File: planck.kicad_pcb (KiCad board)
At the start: 2 copper layers, 113 x 75 mm, 54 parts, among them J1 USB_C_U262-161N-4BVC11, J2 USB_C_U262-161N-4BVC11, SW1 SW_Cherry_MX_1.00u, SW10 SW_Cherry_MX_1.00u, SW11 SW_Cherry_MX_1.00u, SW12 SW_Cherry_MX_1.00u, SW13 SW_Cherry_MX_1.00u, SW14 SW_Cherry_MX_1.00u, SW15 SW_Cherry_MX_1.00u, SW16 SW_Cherry_MX_1.00u, SW17 SW_Cherry_MX_1.00u, SW18 SW_Cherry_MX_1.00u, SW19 SW_Cherry_MX_1.00u, SW2 SW_Cherry_MX_1.00u, SW20 SW_Cherry_MX_1.00u, SW21 SW_Cherry_MX_1.00u, SW22 SW_Cherry_MX_1.00u, SW23 SW_Cherry_MX_1.00u, SW24 SW_Cherry_MX_1.00u, SW3 SW_Cherry_MX_1.00u, SW4 SW_Cherry_MX_1.00u, SW5 SW_Cherry_MX_1.00u, SW6 SW_Cherry_MX_1.00u, SW7 SW_Cherry_MX_1.00u, SW8 SW_Cherry_MX_1.00u, SW9 SW_Cherry_MX_1.00u, U1 RP2040, Y1 32M

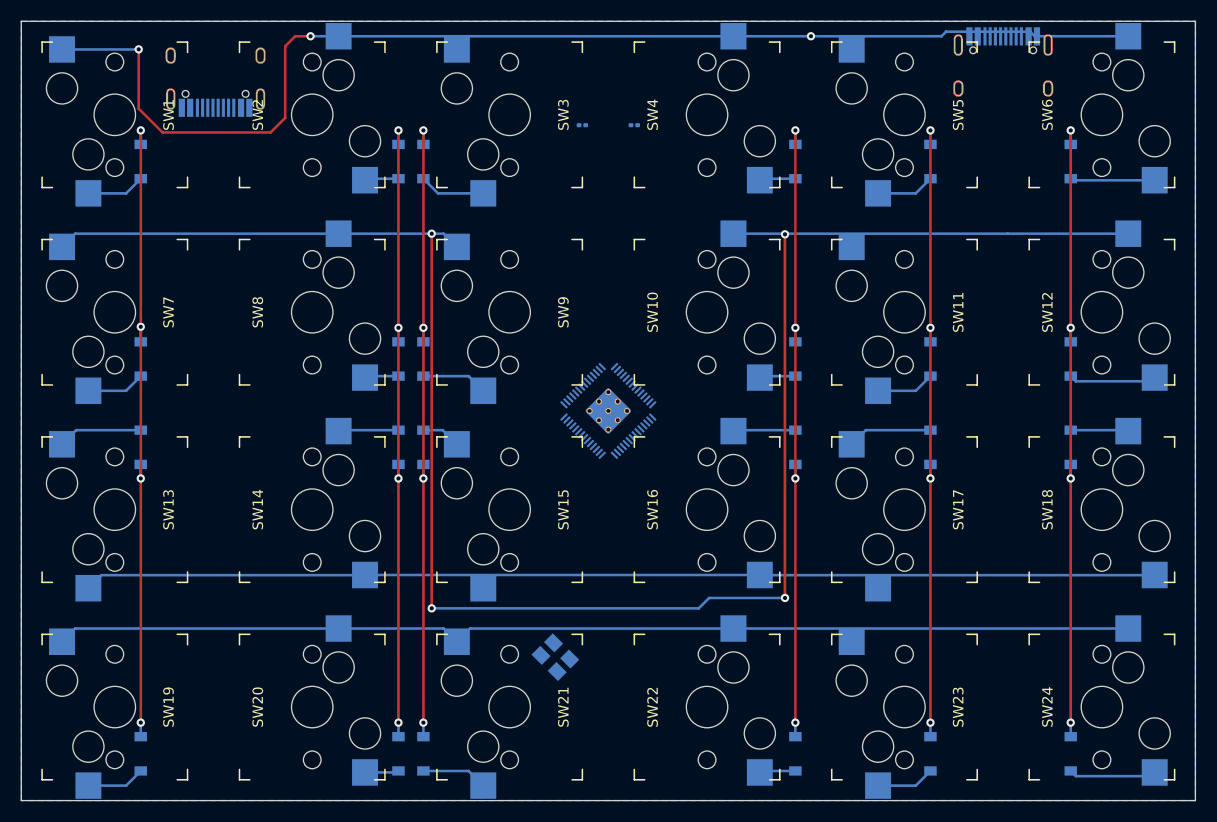
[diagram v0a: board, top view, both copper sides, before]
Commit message: MX version complete
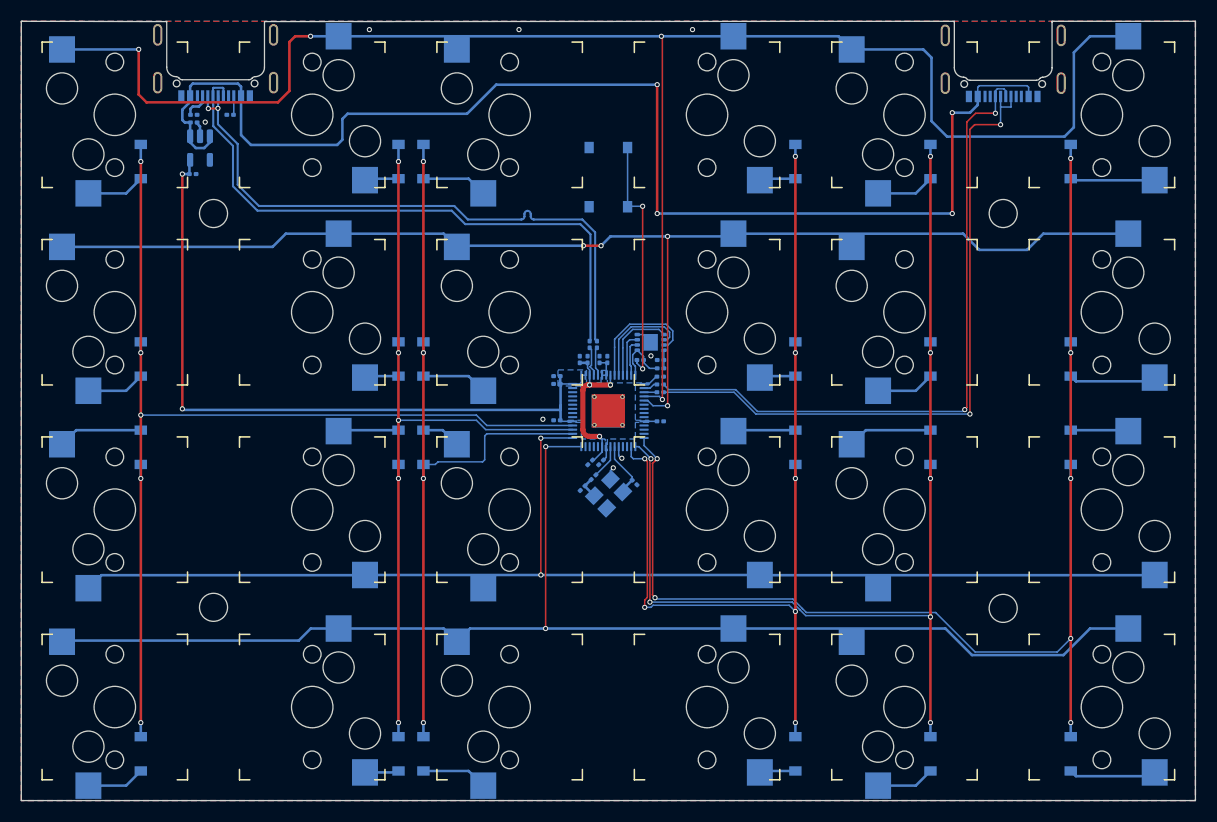
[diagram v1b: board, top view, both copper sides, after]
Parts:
- added C1: 2.2uF ±10% 10V, Resistor_SMD:R_0201_0603Metric, B.Cu at (99.1, 69.7)
- added C10: 100nF ±10% 25V 0201, Resistor_SMD:R_0201_0603Metric, B.Cu at (138.2, 92.5)
- added C11: 100nF ±10% 25V 0201, Resistor_SMD:R_0201_0603Metric, B.Cu at (144.0, 98.5)
- added C12: 100nF ±10% 25V 0201, Resistor_SMD:R_0201_0603Metric, B.Cu at (138.3, 102.5)
- added C13: 100nF ±10% 25V 0201, Resistor_SMD:R_0201_0603Metric, B.Cu at (138.9, 92.5)
- added C14: 1uF ±20% 6.3V 0201, Capacitor_SMD:C_0201_0603Metric, B.Cu at (137.0, 92.5)
- added C15: 100nF ±10% 25V 0201, Resistor_SMD:R_0201_0603Metric, B.Cu at (136.2, 92.5)
- added C16: 100nF ±10% 25V 0201, Resistor_SMD:R_0201_0603Metric, B.Cu at (137.2, 102.5)
- added C2: 2.2uF ±10% 10V, Resistor_SMD:R_0201_0603Metric, B.Cu at (99.0, 74.7)
- added C3: 22pF ±5% 50V 0603, Resistor_SMD:R_0201_0603Metric, B.Cu at (141.5, 104.4)
- added C4: 22pF ±5% 50V 0603, Resistor_SMD:R_0201_0603Metric, B.Cu at (136.5, 104.9)
- added C5: 100nF ±10% 25V 0201, Resistor_SMD:R_0201_0603Metric, B.Cu at (144.0, 92.6)
- added C6: 1uF ±20% 6.3V 0201, Capacitor_SMD:C_0201_0603Metric, B.Cu at (134.1, 94.2)
- added C7: 100nF ±10% 25V 0201, Resistor_SMD:R_0201_0603Metric, B.Cu at (134.1, 94.9)
- added C8: 100nF ±10% 25V 0201, Resistor_SMD:R_0201_0603Metric, B.Cu at (144.0, 94.2)
- added C9: 100nF ±10% 25V 0201, Resistor_SMD:R_0201_0603Metric, B.Cu at (134.1, 98.4)
- added H1: MountingHole, MountingHole:MountingHole_2.7mm_M2.5, F.Cu at (101.0, 78.5)
- added H2: MountingHole, MountingHole:MountingHole_2.7mm_M2.5, F.Cu at (177.0, 78.5)
- added H3: MountingHole, MountingHole:MountingHole_2.7mm_M2.5, F.Cu at (177.0, 116.5)
- added H4: MountingHole, MountingHole:MountingHole_2.7mm_M2.5, F.Cu at (101.0, 116.4)
- added R3: 1kΩ ±1% 50mW 0201, Resistor_SMD:R_0201_0603Metric, B.Cu at (137.6, 103.9)
- added R4: 100Ω ±1% 50mW, Resistor_SMD:R_0201_0603Metric, B.Cu at (144.0, 95.0)
- added R5: 27Ω ±1% 50mW 0201, Resistor_SMD:R_0201_0603Metric, B.Cu at (137.9, 91.1)
- added R6: 27Ω ±1% 50mW 0201, Resistor_SMD:R_0201_0603Metric, B.Cu at (137.2, 91.1)
- added R7: 100Ω ±1% 50mW, Resistor_SMD:R_0201_0603Metric, B.Cu at (144.0, 95.7)
- added R8: 10kΩ ±1% 50mW 0201, Resistor_SMD:R_0201_0603Metric, B.Cu at (144.0, 93.4)
- added R9: 1kΩ ±1% 50mW 0201, Resistor_SMD:R_0201_0603Metric, B.Cu at (142.1, 92.6)
- added SW25: SW_Push, Switches:TSC005A1618A03, B.Cu at (139.0, 75.0)
- added U2: ME6219C33M5G, Package_TO_SOT_SMD:SOT-23-5, B.Cu at (99.7, 72.2)
- added U3: W25Q16JVUXIQ, Package_SON:SON-8-1EP_3x2mm_P0.5mm_EP1.4x1.6mm, B.Cu at (143.1, 90.9)
- D1, D10, D11, D12, D13, D14, D15, D16, D17, D18, D19, D2, D20, D21, D22, D23, D24, D3, D4, D5, D6, D7, D8, D9: value 1N4148W -> 1N4148W,100V 150mA 4ns T4
- J1, J2: footprint josh-connectors:USB_C_U262-161N-4BVC11 -> josh-connectors:USB_C_TYPE-C-31-M-14
- U1: value RP2040 -> RP2040 ARM Cortex-M0 133MHz; footprint RP2040_minimal:RP2040-QFN-56 -> Package_DFN_QFN:QFN-56-1EP_7x7mm_P0.4mm_EP3.2x3.2mm_ThermalVias
- Y1: value 32M -> 32MHz ±10ppm 20pF SMD3225-4P
- moved R2 38.9 mm to (102.6, 69.0), turned to 180 degrees
- moved R1 37.4 mm to (99.1, 69.0), turned to 0 degrees
- moved Y1 16.5 mm to (139.0, 105.5), turned to -135 degrees
- moved J2 0.85 mm to (101.2, 64.3)
- moved J1 0.22 mm to (177.0, 64.4), turned to 0 degrees
- turned U1 to 180 degrees
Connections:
- net /d+ renamed /D-
- net /d- renamed /D+
- U1 pad 1: unconnected-(U1-Pad1) -> /V3V3
- U1 pad 10: unconnected-(U1-Pad10) -> /V3V3
- U1 pad 14: unconnected-(U1-Pad14) -> c6
- U1 pad 15: unconnected-(U1-Pad15) -> c5
- U1 pad 16: unconnected-(U1-Pad16) -> c4
- U1 pad 19: unconnected-(U1-Pad19) -> GND
- U1 pad 2: unconnected-(U1-Pad2) -> /tx0
- U1 pad 20: unconnected-(U1-Pad20) -> /X32MI
- U1 pad 21: unconnected-(U1-Pad21) -> /X32MO
- U1 pad 22: unconnected-(U1-Pad22) -> /V3V3
- U1 pad 23: unconnected-(U1-Pad23) -> /V1V1
- U1 pad 28: unconnected-(U1-Pad28) -> r4
- U1 pad 29: unconnected-(U1-Pad29) -> r3
- U1 pad 3: unconnected-(U1-Pad3) -> /rx0
- U1 pad 30: unconnected-(U1-Pad30) -> c3
- U1 pad 31: unconnected-(U1-Pad31) -> c2
- U1 pad 32: unconnected-(U1-Pad32) -> c1
- U1 pad 33: unconnected-(U1-Pad33) -> /V3V3
- U1 pad 4: unconnected-(U1-Pad4) -> r1
- U1 pad 42: unconnected-(U1-Pad42) -> /V3V3
- U1 pad 43: unconnected-(U1-Pad43) -> /V3V3
- U1 pad 44: unconnected-(U1-Pad44) -> /V3V3
- U1 pad 45: unconnected-(U1-Pad45) -> /V1V1
- U1 pad 46: unconnected-(U1-Pad46) -> Net-(R6-Pad1)
- U1 pad 47: unconnected-(U1-Pad47) -> Net-(R5-Pad1)
- U1 pad 48: unconnected-(U1-Pad48) -> /V3V3
- U1 pad 49: unconnected-(U1-Pad49) -> /V3V3
- U1 pad 5: unconnected-(U1-Pad5) -> r2
- U1 pad 50: unconnected-(U1-Pad50) -> /V1V1
- U1 pad 51: unconnected-(U1-Pad51) -> /QSPI_SD3
- U1 pad 52: unconnected-(U1-Pad52) -> /QSPI_CLK
- U1 pad 53: unconnected-(U1-Pad53) -> /QSPI_SD0
- U1 pad 54: unconnected-(U1-Pad54) -> /QSPI_SD2
- U1 pad 55: unconnected-(U1-Pad55) -> /QSPI_SD1
- U1 pad 56: unconnected-(U1-Pad56) -> /QSPI_SS
- U1 pad 57: unconnected-(U1-Pad57) -> GND
- Y1 pad 3: /X32MO -> Net-(C4-Pad1)
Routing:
- net /VBUS: track 0.00 -> 123.6 mm, vias 0 -> 4
- net /V3V3: track 0.00 -> 76.6 mm, vias 0 -> 2
- net Net-(J1-PadA6): track 0.00 -> 65.6 mm, vias 0 -> 2
- net Net-(J1-PadA7): track 0.00 -> 64.9 mm, vias 0 -> 2
- net /D-: track 0.00 -> 59.5 mm, vias 0 -> 2
- net /D+: track 0.00 -> 58.6 mm
- net r2: track 182.5 -> 124.3 mm
- net c6: track 62.4 -> 118.3 mm, vias 4 -> 7
- net r1: track 118.0 -> 165.4 mm, vias 3 -> 4
- net c5: track 62.4 -> 102.8 mm, vias 4 -> 7
- net c1: track 62.5 -> 101.4 mm, vias 4 -> 5
- net c4: track 62.4 -> 91.1 mm, vias 4 -> 7
- net Net-(R9-Pad1): track 0.00 -> 23.9 mm, vias 0 -> 2
- net r4: track 104.2 -> 127.3 mm, vias 0 -> 2
- net r3: track 103.2 -> 119.4 mm, vias 0 -> 2
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- added copper zone on B.Cu, net /V3V3
- added copper zone on F.Cu, net GND
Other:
- outline, holes or cut-outs redrawn
- board text added: "boot"
